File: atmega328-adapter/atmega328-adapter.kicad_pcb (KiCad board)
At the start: 2 copper layers, 21.3 x 36.6 mm, 3 parts, among them U4 ATmega168A-A

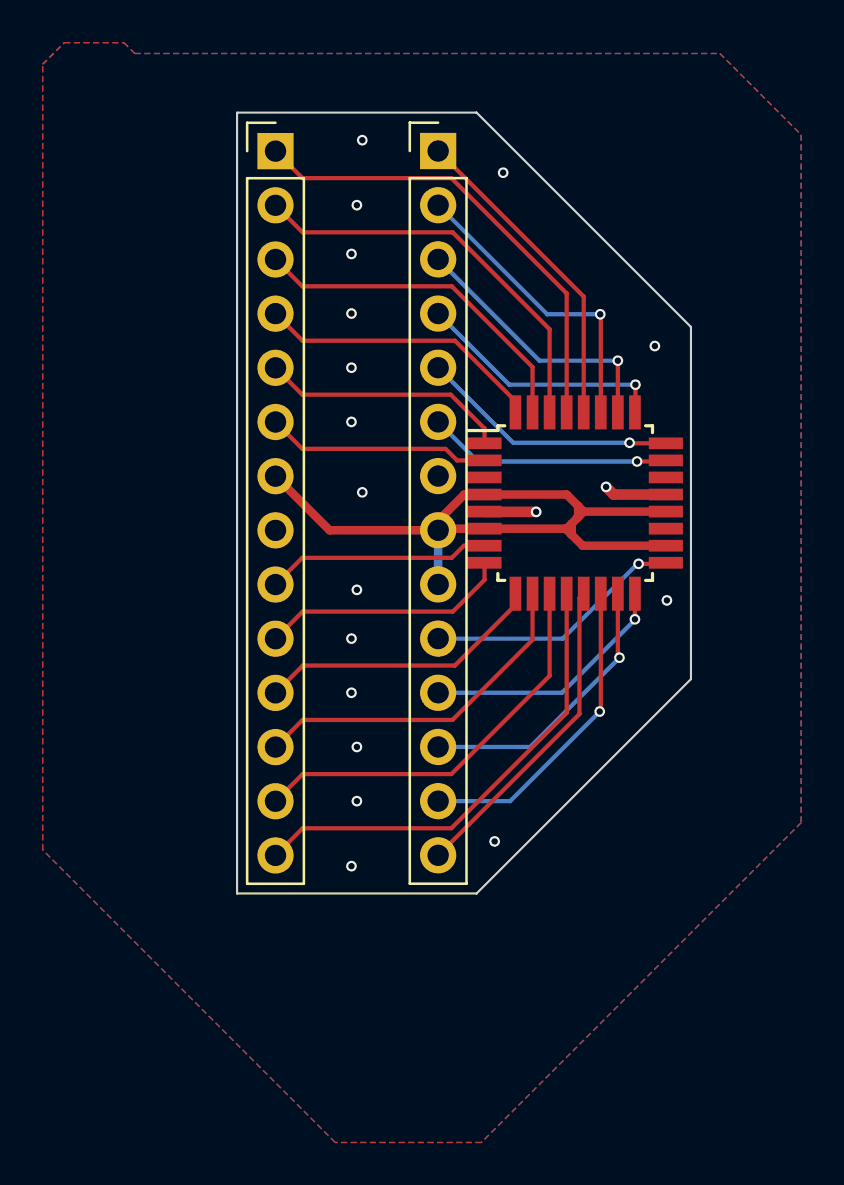
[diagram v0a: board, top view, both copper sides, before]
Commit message: updated adapter
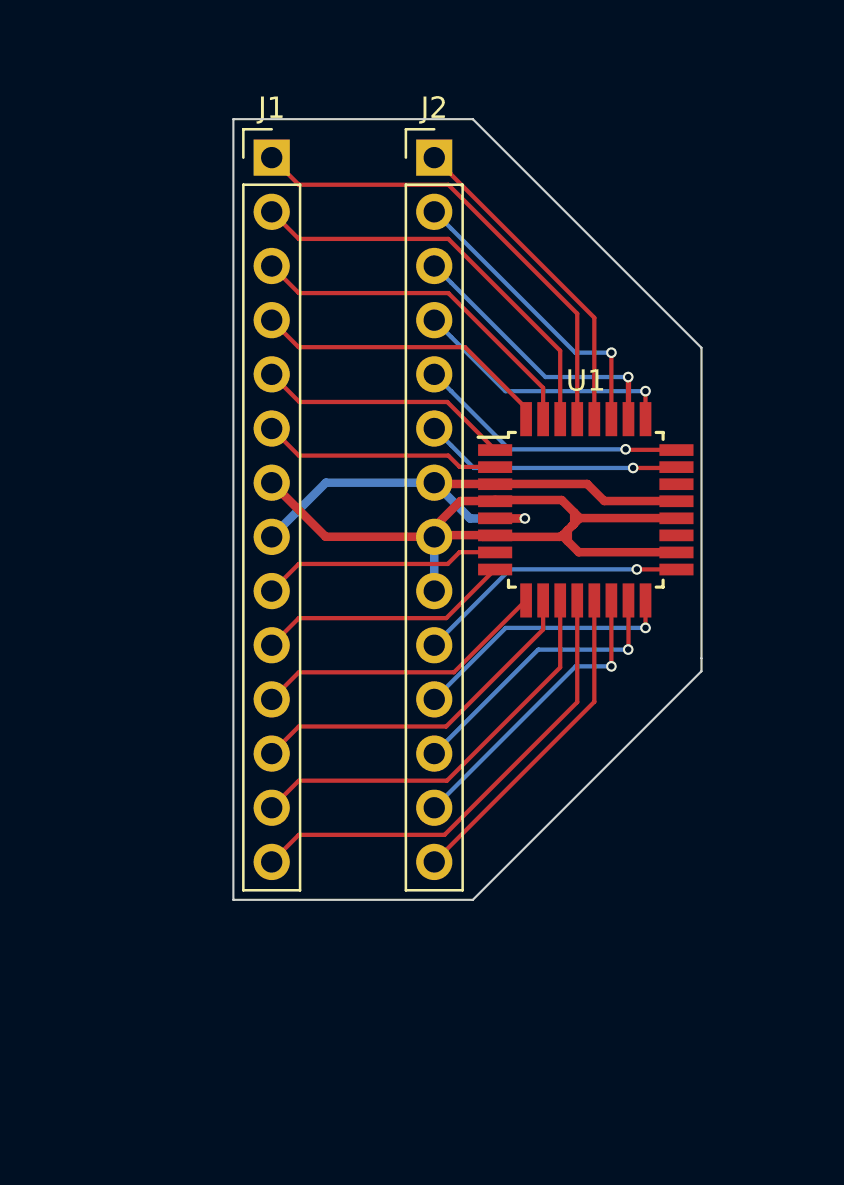
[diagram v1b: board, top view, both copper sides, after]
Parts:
- removed REF** (x2): PinHeader_1x14_P2.54mm_Vertical, Connector_PinHeader_2.54mm:PinHeader_1x14_P2.54mm_Vertical
- removed U4: ATmega168A-A, Package_QFP:TQFP-32_7x7mm_P0.8mm
- added J1: Conn_01x14, Connector_PinHeader_2.54mm:PinHeader_1x14_P2.54mm_Vertical, F.Cu at (114.9, 50.4)
- added J2: Conn_01x14, Connector_PinHeader_2.54mm:PinHeader_1x14_P2.54mm_Vertical, F.Cu at (122.5, 50.4)
- added U1: ATmega168A-A, Package_QFP:TQFP-32_7x7mm_P0.8mm, F.Cu at (129.7, 67.0)
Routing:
- net (no net): track 373.3 -> 0.00 mm, vias 28 -> 0
- net +5V: track 0.00 -> 38.6 mm
- net GND: track 0.00 -> 26.0 mm, vias 0 -> 1
- net /RESET: track 0.00 -> 22.3 mm
- net /PB0: track 0.00 -> 22.2 mm
- net /PD0: track 0.00 -> 19.4 mm
- net /PD7: track 0.00 -> 19.4 mm
- net /PC5: track 0.00 -> 17.2 mm
- net /PD1: track 0.00 -> 16.6 mm
- net /PD6: track 0.00 -> 16.5 mm
- net /PB1: track 0.00 -> 15.4 mm
- net /CS: track 0.00 -> 14.2 mm, vias 0 -> 1
- net /PC4: track 0.00 -> 14.2 mm, vias 0 -> 1
- net /PD2: track 0.00 -> 14.1 mm
- net /PD5: track 0.00 -> 13.9 mm
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- removed copper zone on B.Cu, net (none)
- removed copper zone on F.Cu, net (none)
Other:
- board size 21.3 x 36.6 mm -> 21.9 x 36.6 mm
